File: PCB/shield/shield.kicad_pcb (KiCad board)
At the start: 2 copper layers, 113.1 x 80.1 mm, 19 parts, among them J1 QTR-8A, J10 ESP32_left_m, J11 ESP32_right_m, J13 Conn_01x06, J14 Domino, J15 Domino, J2 QMC5883L, J3 Servo, J4 Domino, J5 Joystick, J6 OLED, J8 ESP32_left_f, J9 ESP32_right_f, U1 YAAJ_DCDC_StepDown_LM2596

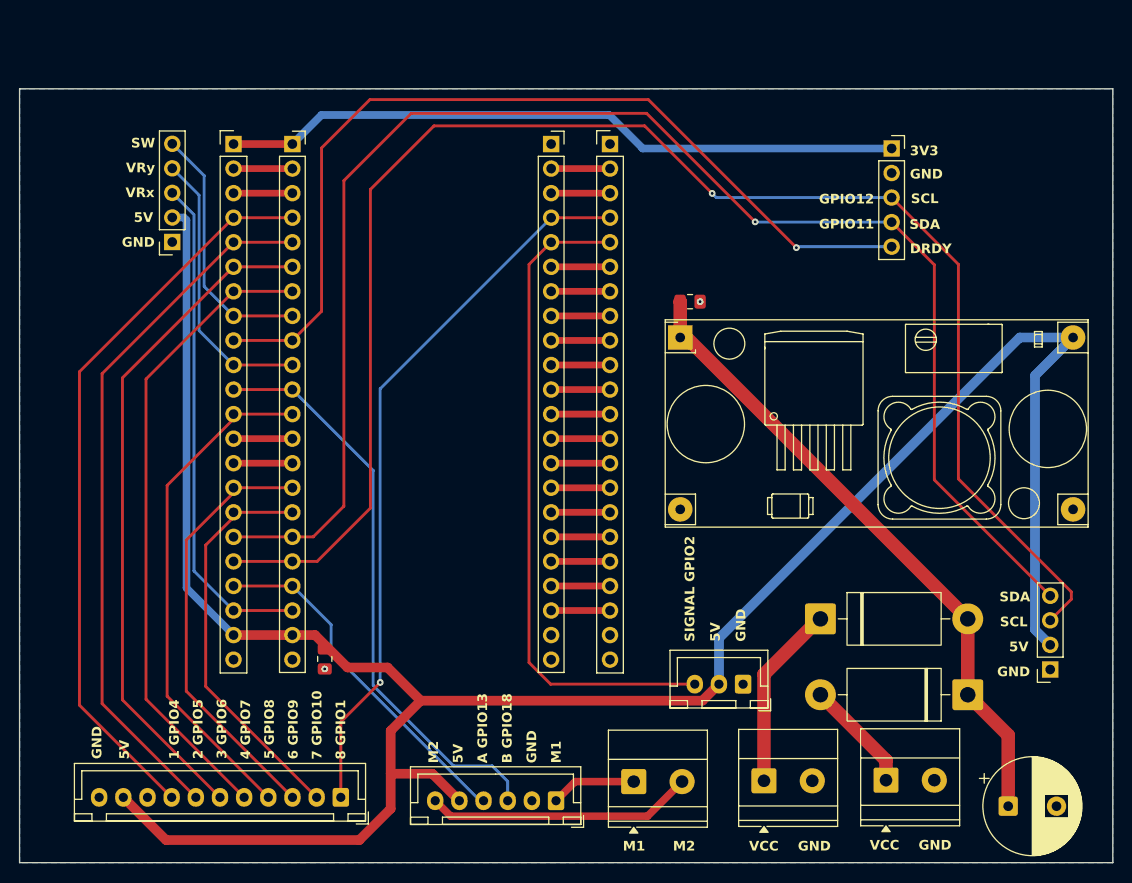
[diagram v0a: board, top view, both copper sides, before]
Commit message: wip: commit to change workplace
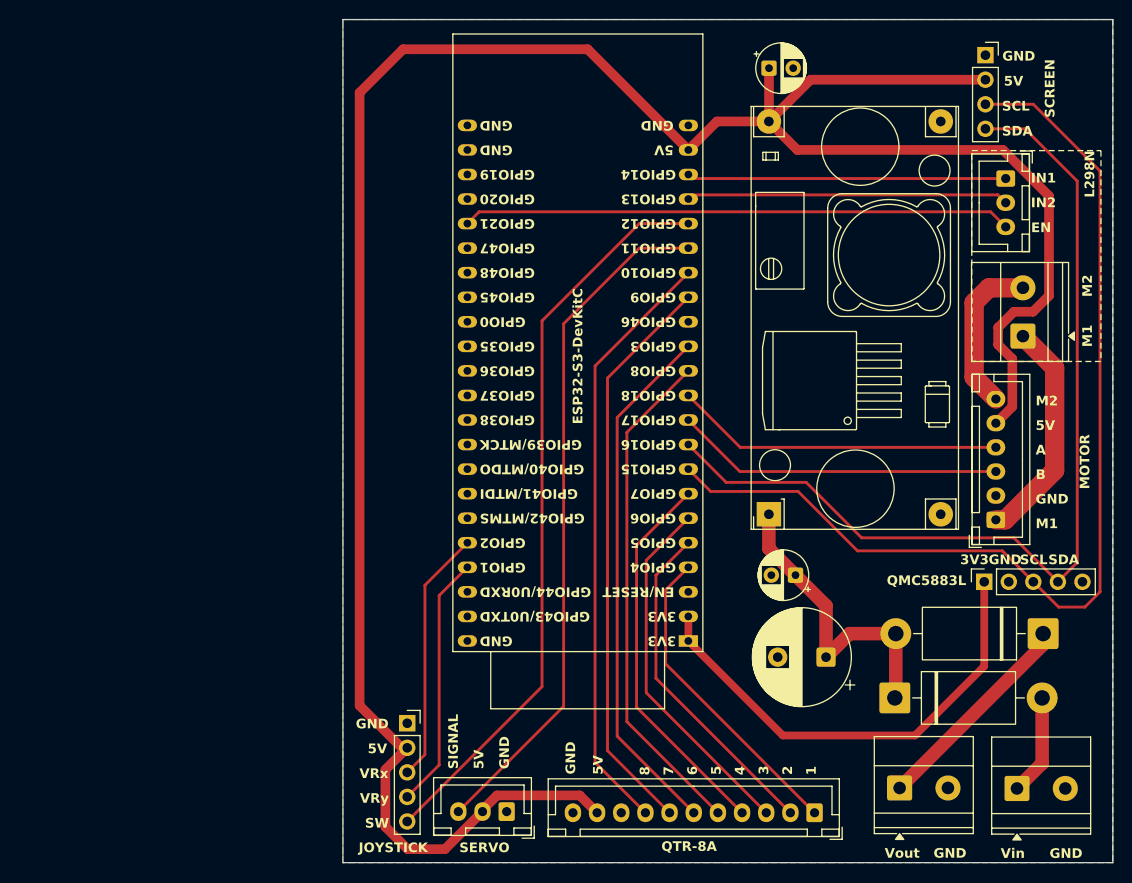
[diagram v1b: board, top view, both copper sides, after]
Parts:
- removed J10: ESP32_left_m, Connector_PinHeader_2.54mm:PinHeader_1x22_P2.54mm_Vertical
- removed J11: ESP32_right_m, Connector_PinHeader_2.54mm:PinHeader_1x22_P2.54mm_Vertical
- removed J8: ESP32_left_f, Connector_PinSocket_2.54mm:PinSocket_1x22_P2.54mm_Vertical
- removed J9: ESP32_right_f, Connector_PinSocket_2.54mm:PinSocket_1x22_P2.54mm_Vertical
- added J7: L298N, Connector_JST:JST_XH_B3B-XH-A_1x03_P2.50mm_Vertical, F.Cu at (189.6, 76.3)
- added U2: ESP32-S3-DevKitC, PCM_Espressif:ESP32-S3-DevKitC, F.Cu at (156.8, 124.1)
- C3, C5: footprint Capacitor_SMD:C_0805_2012Metric_Pad1.18x1.45mm_HandSolder -> Capacitor_THT:CP_Radial_D5.0mm_P2.50mm
- moved C5 76.5 mm to (165.1, 64.9), turned to 0 degrees
- moved J6 63.9 mm to (187.5, 63.5), turned to 0 degrees
- moved J14 61.2 mm to (191.4, 92.6), turned to 90 degrees
- moved J5 55.4 mm to (127.7, 132.6), turned to 0 degrees
- moved J13 54.0 mm to (188.6, 111.6), turned to 90 degrees
- moved J1 49.0 mm to (169.8, 141.9)
- moved J2 45.8 mm to (187.4, 118.0), turned to 90 degrees
- moved C3 30.3 mm to (167.9, 117.3), turned to 180 degrees
- moved J3 27.8 mm to (138.0, 141.8)
- moved C1 24.3 mm to (171.0, 125.8), turned to 180 degrees
- moved U1 20.5 mm to (165.1, 111.0), turned to 90 degrees
- moved J15 14.1 mm to (178.6, 139.3)
- moved J4 13.6 mm to (190.8, 139.4)
- moved D2 11.2 mm to (178.1, 130.0)
- moved D1 10.0 mm to (193.5, 123.4)
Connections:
- net Net-(J13-Pin_1) renamed /M1
- net Net-(J13-Pin_6) renamed /M2
- D1 pad 1: VCC -> Net-(D1-K)
- D1 pad 2: Net-(D1-A) -> VCC
- D2 pad 1: Net-(D2-K) -> VCC
- D2 pad 2: VCC -> Net-(D2-A)
- J1 pad 1: /GPIO1 -> /GPIO4
- J1 pad 2: /GPIO10 -> /GPIO5
- J1 pad 3: /GPIO9 -> /GPIO6
- J1 pad 4: /GPIO8 -> /GPIO7
- J1 pad 5: /GPIO7 -> /GPIO8
- J1 pad 6: /GPIO6 -> /GPIO3
- J1 pad 7: /GPIO5 -> /GPIO9
- J1 pad 8: /GPIO4 -> /GPIO10
- J13 pad 3: /GPIO18 -> /GPIO17
- J13 pad 4: /GPIO13 -> /GPIO18
- J15 pad 1: Net-(D2-K) -> Net-(D1-K)
- J2 pad 3: /GPIO12+SCL -> /GPIO15
- J2 pad 4: /GPIO11+SDA -> /GPIO16
- J2 pad 5: /GPIO16 -> unconnected-(J2-Pin_5-Pad5)
- J3 pad 3: /GPIO2 -> /GPIO11
- J4 pad 1: Net-(D1-A) -> Net-(D2-A)
- J5 pad 3: /GPIO14 -> /GPIO2
- J5 pad 4: /GPIO17 -> /GPIO1
- J5 pad 5: /GPIO15 -> /GPIO12
- J6 pad 3: /GPIO12+SCL -> /GPIO15
- J6 pad 4: /GPIO11+SDA -> /GPIO16
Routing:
- net /GPIO12+SCL: track 161.5 -> 0.00 mm, vias 1 -> 0
- net /GPIO11+SDA: track 156.1 -> 0.00 mm, vias 1 -> 0
- net /GPIO15: track 26.5 -> 107.4 mm
- net /GPIO12: track 0.00 -> 76.9 mm
- net /GPIO11: track 0.00 -> 71.1 mm
- net /GPIO21: track 0.00 -> 56.8 mm
- net /GPIO3: track 0.00 -> 54.6 mm
- net /GPIO1: track 75.1 -> 26.3 mm, vias 1 -> 0
- net /GPIO4: track 76.6 -> 32.8 mm
- net /GPIO2: track 68.6 -> 26.3 mm
- net /GPIO5: track 73.2 -> 35.1 mm
- net VCC: track 66.6 -> 32.2 mm
- net /GPIO6: track 69.9 -> 37.4 mm
- net /GPIO7: track 66.4 -> 39.8 mm
- net /GPIO18: track 60.2 -> 34.0 mm
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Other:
- board size 113.1 x 80.1 mm -> 79.7 x 87.2 mm
- board text added: "1"
- board text added: "2"
- board text added: "3"
- board text added: "4"
- board text added: "5"
- board text added: "6"
- board text added: "7"
- board text added: "8"
- board text added: "A"
- board text added: "B"
- board text added: "EN"
- board text added: "IN1"
- board text added: "IN2"
- board text added: "JOYSTICK"
- board text added: "L298N"
- board text added: "MOTOR"
- board text added: "QMC5883L"
- board text added: "QTR-8A"
- board text added: "SCREEN"
- board text added: "SERVO"
- board text added: "SIGNAL"
- board text added: "Vin"
- board text added: "Vout"
- board text removed: "1 GPIO4"
- board text removed: "2 GPIO5"
- board text removed: "3 GPIO6"
- board text removed: "4 GPIO7"
- board text removed: "5 GPIO8"
- board text removed: "6 GPIO9"
- board text removed: "7 GPIO10"
- board text removed: "8 GPIO1"
- board text removed: "A GPIO13"
- board text removed: "B GPIO18"
- board text removed: "DRDY"
- board text removed: "GPIO11"
- board text removed: "GPIO12"
- board text removed: "SIGNAL GPIO2"
- board text removed: "VCC"
